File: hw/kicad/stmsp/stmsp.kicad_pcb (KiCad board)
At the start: 4 copper layers, 42 x 42 mm, 135 parts, among them J1 CONN_02X05, P1 USB_OTG, P2 CONN_01X04, P3 CONN_01X04, P4 CONN_01X02, P5 CONN_01X06, P6 CONN_01X02, Q1 Q_NJFET_GSD, Q2 Q_NJFET_GSD, T1 testpoint, T2 testpoint, T3 testpoint, T4 testpoint, T5 testpoint, U1 USBLC6-4SC6, U10 TLE5012, U2 L6206Q, U3 STM32F303CBTx, U4 USBLC6-4SC6, U5 MCP16331, U6 MIC5504-3.3YM5, U7 TLE5012, U8 SN65176B, U9 SN65176B, Y1 8M

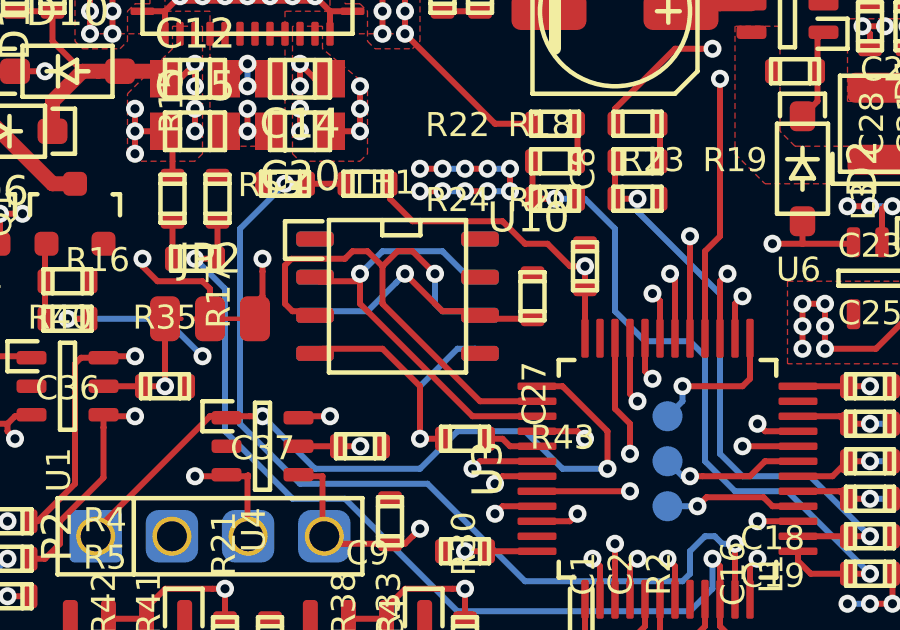
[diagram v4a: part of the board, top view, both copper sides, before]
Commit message: stmsp
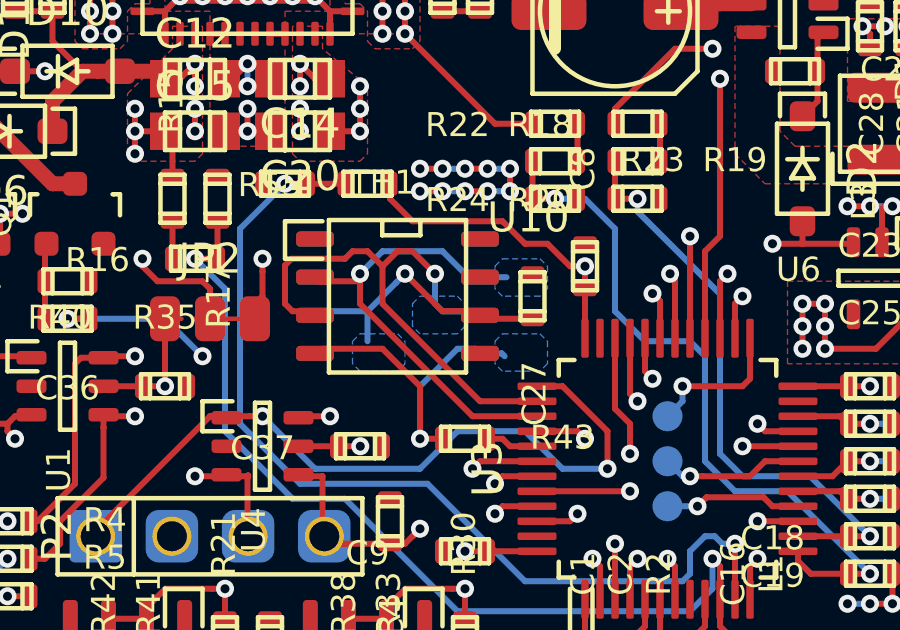
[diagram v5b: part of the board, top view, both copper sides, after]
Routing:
- net Net-(C27-Pad1): track 22.0 -> 23.0 mm
- net /SCK: track 14.7 -> 15.6 mm
- net /MOSI: track 11.8 -> 12.7 mm
- added copper zone on B.Cu, net /CSQ
- added copper zone on B.Cu, net /MOSI
- added copper zone on B.Cu, net /SCK
- added copper zone on B.Cu, net Net-(C27-Pad1)
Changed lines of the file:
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@@
     (thickness 1.6)
     (drawings 20)
-    (tracks 1234)
+    (tracks 1238)
     (zones 0)
     (modules 135)
@@
   (segment (start 85 63.5) (end 85 62.4) (width 0.2) (layer F.Cu) (net 16) (status 30))
   (segment (start 85 62.4) (end 85.2 62.2) (width 0.2) (layer F.Cu) (net 16) (status 30))
+  (segment (start 70 71.5) (end 70 72.5) (width 0.2) (layer B.Cu) (net 17))
   (segment (start 62.5 69.75) (end 62.5 70) (width 0.2) (layer F.Cu) (net 17))
   (segment (start 62.5 70) (end 63 70.5) (width 0.2) (layer F.Cu) (net 17))
@@
   (segment (start 69.25 83.25) (end 68.095 82.095) (width 0.2) (layer F.Cu) (net 60) (status 20))
   (segment (start 68.095 82.095) (end 68.095 81.75) (width 0.2) (layer F.Cu) (net 60) (status 30))
+  (segment (start 73.75 72.905) (end 74.475 72.905) (width 0.2) (layer B.Cu) (net 61))
+  (segment (start 74.475 72.905) (end 74.57 73) (width 0.2) (layer B.Cu) (net 61))
   (segment (start 72.5 75.75) (end 71.75 75.75) (width 0.2) (layer F.Cu) (net 61))
   (segment (start 71.75 75.75) (end 71.75 74) (width 0.2) (layer B.Cu) (net 61))
@@
   (segment (start 68.75 73) (end 68.655 72.905) (width 0.2) (layer F.Cu) (net 61) (status 30))
   (segment (start 68.655 72.905) (end 68.25 72.905) (width 0.2) (layer F.Cu) (net 61) (status 30))
+  (segment (start 73.75 70.365) (end 74.635 70.365) (width 0.2) (layer B.Cu) (net 62))
   (segment (start 69.75 70.25) (end 70.5 69.5) (width 0.2) (layer B.Cu) (net 62))
   (segment (start 70.5 69.5) (end 72.5 69.5) (width 0.2) (layer B.Cu) (net 62))
@@
       )
     )
+  )
+  (zone (net 61) (net_name /MOSI) (layer B.Cu) (hatch edge 0.508)
+    (priority 1)
+    (connect_pads yes (clearance 0.25))
+    (min_thickness 0.254)
+    (fill yes (arc_segments 16) (thermal_gap 0.508) (thermal_bridge_width 0.508))
+    (polygon
+      (pts
+        (xy 74.25 72.5) (xy 74.5 72.25) (xy 75.75 72.25) (xy 76 72.5) (xy 76 73.25)
+        (xy 75.75 73.5) (xy 74.5 73.5) (xy 74.25 73.25)
+      )
+    )
+  )
+  (zone (net 63) (net_name /CSQ) (layer B.Cu) (hatch edge 0.508)
+    (priority 1)
+    (connect_pads yes (clearance 0.25))
+    (min_thickness 0.254)
+    (fill yes (arc_segments 16) (thermal_gap 0.508) (thermal_bridge_width 0.508))
+    (polygon
+      (pts
+        (xy 71.5 71.25) (xy 71.75 71) (xy 73 71) (xy 73.25 71.25) (xy 73.25 72)
+        (xy 73 72.25) (xy 71.75 72.25) (xy 71.5 72)
+      )
+    )
+  )
+  (zone (net 62) (net_name /SCK) (layer B.Cu) (hatch edge 0.508)
+    (priority 1)
+    (connect_pads yes (clearance 0.25))
+    (min_thickness 0.254)
+    (fill yes (arc_segments 16) (thermal_gap 0.508) (thermal_bridge_width 0.508))
+    (polygon
+      (pts
+        (xy 74.25 70) (xy 74.5 69.75) (xy 75.75 69.75) (xy 76 70) (xy 76 70.75)
+        (xy 75.75 71) (xy 74.5 71) (xy 74.25 70.75)
+      )
+    )
+  )
+  (zone (net 0) (net_name "") (layer B.Mask) (hatch edge 0.508)
+    (priority 1)
+    (connect_pads yes (clearance 0.25))
+    (min_thickness 0.254)
+    (fill yes (arc_segments 16) (thermal_gap 0.508) (thermal_bridge_width 0.508))
+    (polygon
+      (pts
+        (xy 75.75 72.25) (xy 76 72.5) (xy 76 73.25) (xy 75.75 73.5) (xy 74.5 73.5)
+        (xy 74.25 73.25) (xy 74.25 72.5) (xy 74.5 72.25)
+      )
+    )
+  )
+  (zone (net 0) (net_name "") (layer B.Mask) (hatch edge 0.508)
+    (priority 1)
+    (connect_pads yes (clearance 0.25))
+    (min_thickness 0.254)
+    (fill yes (arc_segments 16) (thermal_gap 0.508) (thermal_bridge_width 0.508))
+    (polygon
+      (pts
+        (xy 75.75 69.75) (xy 76 70) (xy 76 70.75) (xy 75.75 71) (xy 74.5 71)
+        (xy 74.25 70.75) (xy 74.25 70) (xy 74.5 69.75)
+      )
+    )
+  )
+  (zone (net 0) (net_name "") (layer B.Mask) (hatch edge 0.508)
+    (priority 1)
+    (connect_pads yes (clearance 0.25))
+    (min_thickness 0.254)
+    (fill yes (arc_segments 16) (thermal_gap 0.508) (thermal_bridge_width 0.508))
+    (polygon
+      (pts
+        (xy 73 71) (xy 73.25 71.25) (xy 73.25 72) (xy 73 72.25) (xy 71.75 72.25)
+        (xy 71.5 72) (xy 71.5 71.25) (xy 71.75 71)
+      )
+    )
+  )
+  (zone (net 17) (net_name "Net-(C27-Pad1)") (layer B.Cu) (hatch edge 0.508)
+    (priority 1)
+    (connect_pads yes (clearance 0.25))
+    (min_thickness 0.254)
+    (fill yes (arc_segments 16) (thermal_gap 0.508) (thermal_bridge_width 0.508))
+    (polygon
+      (pts
+        (xy 69.5 72.5) (xy 69.75 72.25) (xy 71 72.25) (xy 71.25 72.5) (xy 71.25 73.25)
+        (xy 71 73.5) (xy 69.75 73.5) (xy 69.5 73.25)
+      )
+    )
+  )
+  (zone (net 0) (net_name "") (layer B.Mask) (hatch edge 0.508)
+    (priority 1)
+    (connect_pads yes (clearance 0.25))
+    (min_thickness 0.254)
+    (fill yes (arc_segments 16) (thermal_gap 0.508) (thermal_bridge_width 0.508))
+    (polygon
+      (pts
+        (xy 71 72.25) (xy 71.25 72.5) (xy 71.25 73.25) (xy 71 73.5) (xy 69.75 73.5)
+        (xy 69.5 73.25) (xy 69.5 72.5) (xy 69.75 72.25)
+      )
+    )
+  )
+  (zone (net 0) (net_name "") (layer B.Mask) (hatch edge 0.508)
+    (priority 1)
+    (connect_pads yes (clearance 0.25))
+    (min_thickness 0.254)
+    (fill yes (arc_segments 16) (thermal_gap 0.508) (thermal_bridge_width 0.508))
+    (polygon
+      (pts
+        (xy 71 67.75) (xy 71.25 68) (xy 71.25 68.75) (xy 71 69) (xy 69.75 69)
+        (xy 69.5 68.75) (xy 69.5 68) (xy 69.75 67.75)
+      )
+    )

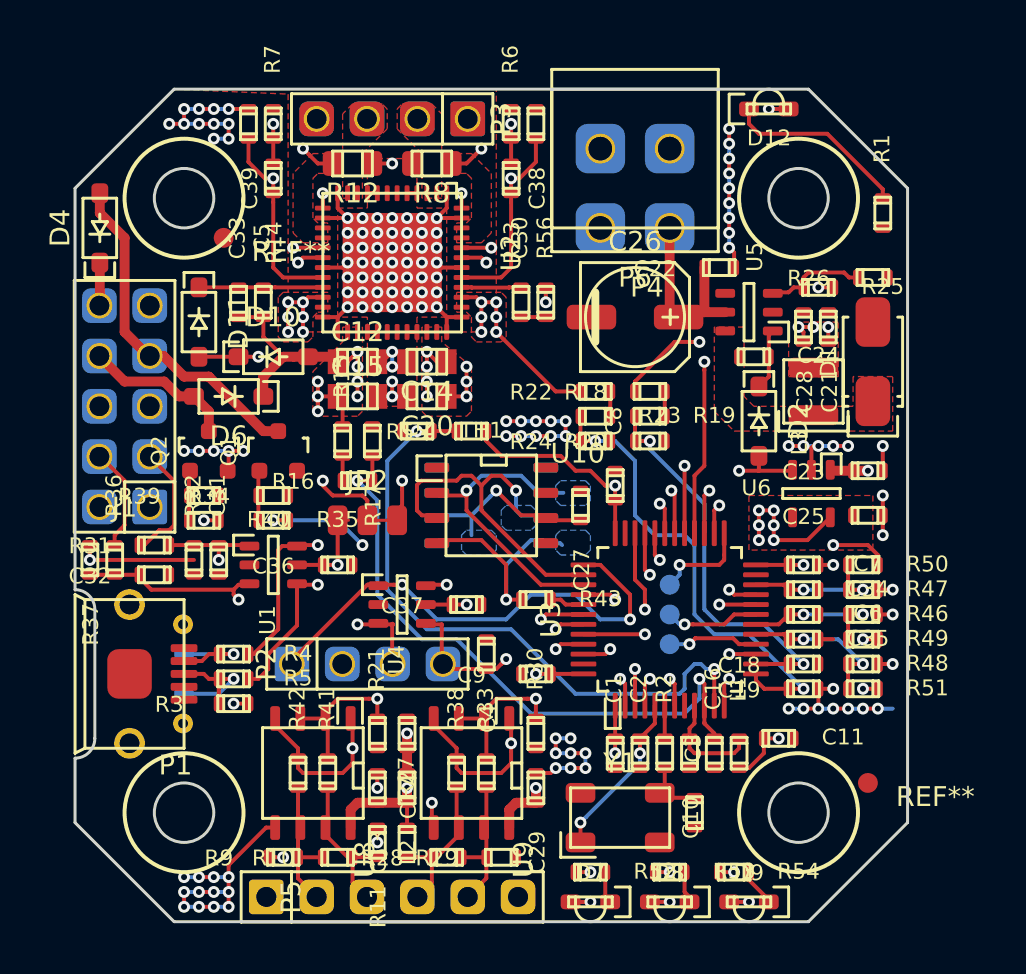
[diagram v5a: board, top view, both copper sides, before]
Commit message: stmsp
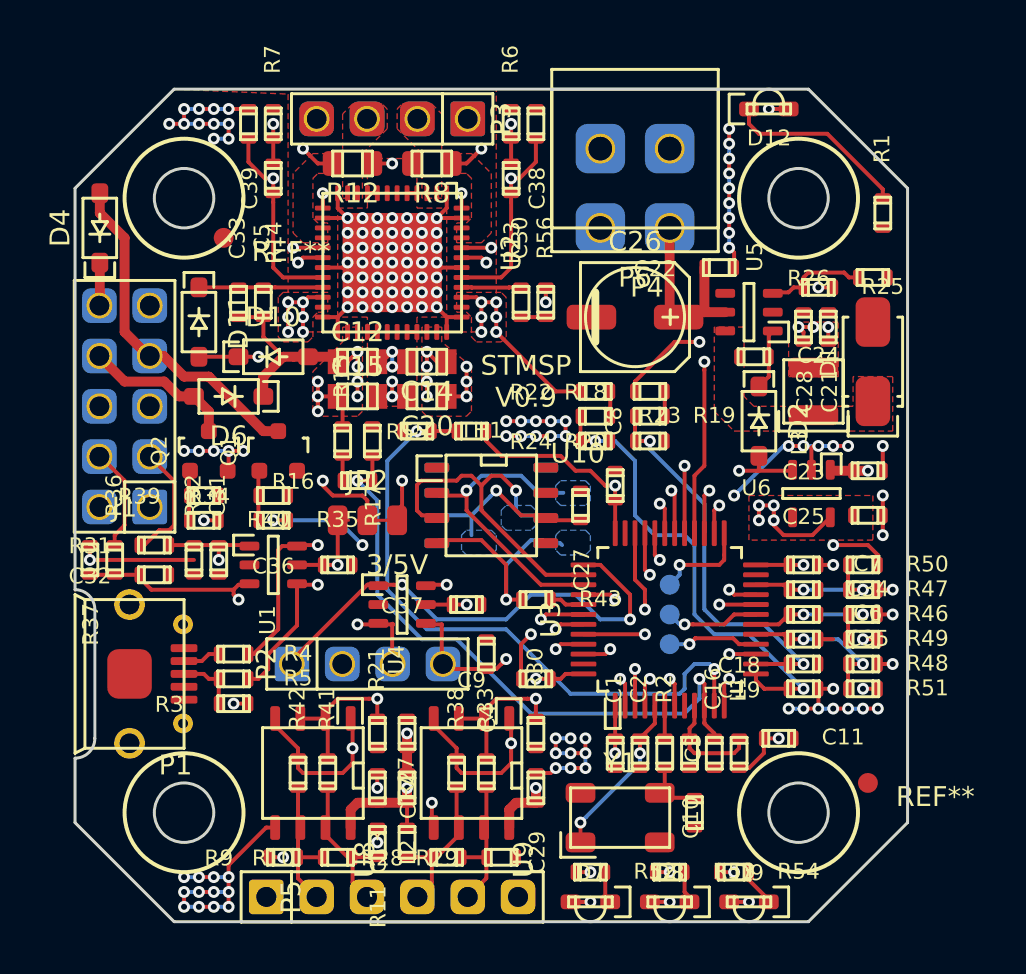
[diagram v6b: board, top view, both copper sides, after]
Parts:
- removed T4, T5: testpoint, stmbl:Measurement_Point_Round-SMD-Pad_Small
- added REF**: STMSP_LOGO, stmbl:STMSP_LOGO, B.Cu at (78.5, 83.8)
- moved C9 0.25 mm to (73.2, 79.8)
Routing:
- net GND: track 177.3 -> 183.5 mm, vias 132 -> 135
- net Net-(P1-Pad3): track 6.16 -> 2.85 mm, vias 1 -> 0
- net Net-(P1-Pad2): track 4.89 -> 1.64 mm, vias 1 -> 0
- net +3V3: track 47.6 -> 46.5 mm, vias 19 -> 17
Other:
- board text added: "+ DC - 12-48V"
- board text added: "0 A B"
- board text added: "0V B/TX A/RX C VP"
- board text added: "1A 2A 1B 2B"
- board text added: "3/5V"
- board text added: "5V A1 B1 A0 B0 0V"
- board text added: "CL 0V IO RS"
- board text added: "DC O1 0V I1 5V DC O0 0V I0 5V"
- board text added: "STMSP V0.9"
- board text added: "STMSP V0.9 (GITHASH) github.com/rene-dev/stmbl"
